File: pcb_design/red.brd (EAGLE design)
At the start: 160 x 100 mm, 6 parts, among them J1 4P-2.0, J2 4P-2.0

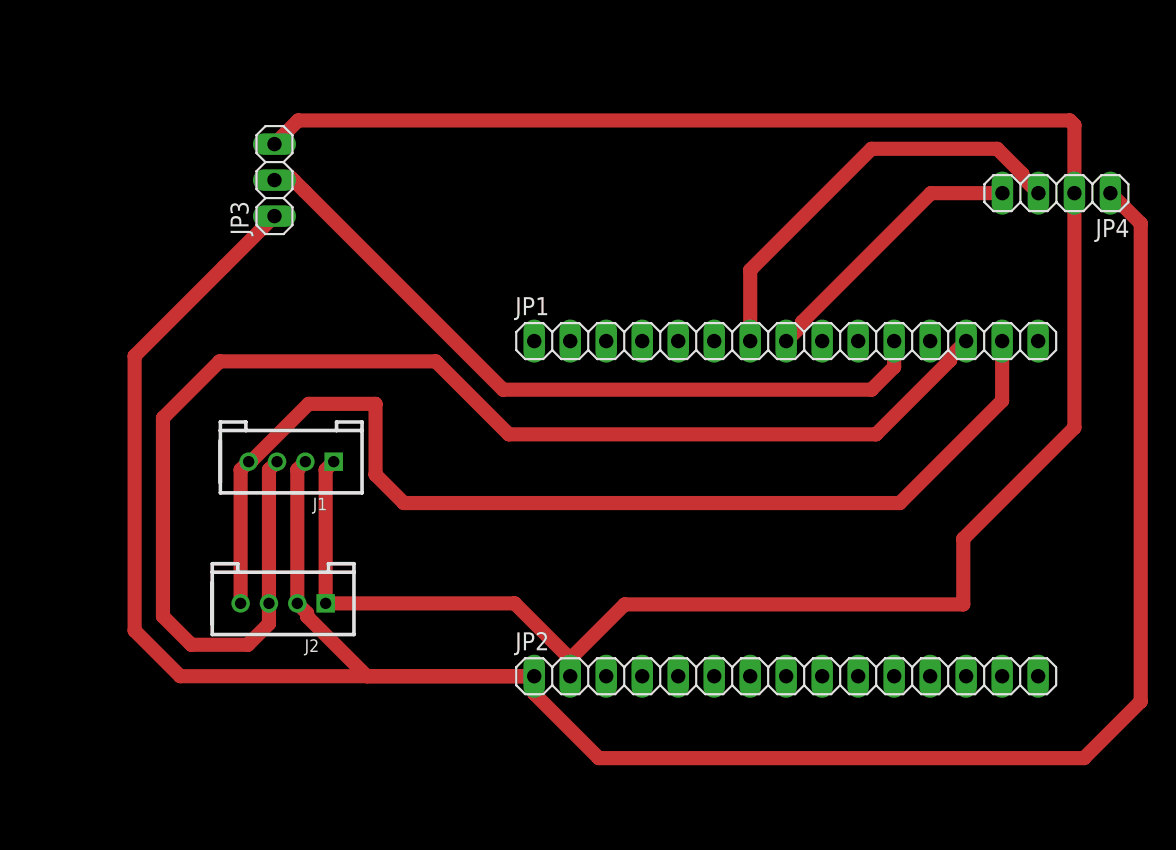
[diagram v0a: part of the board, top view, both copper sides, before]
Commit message: added latest combined data
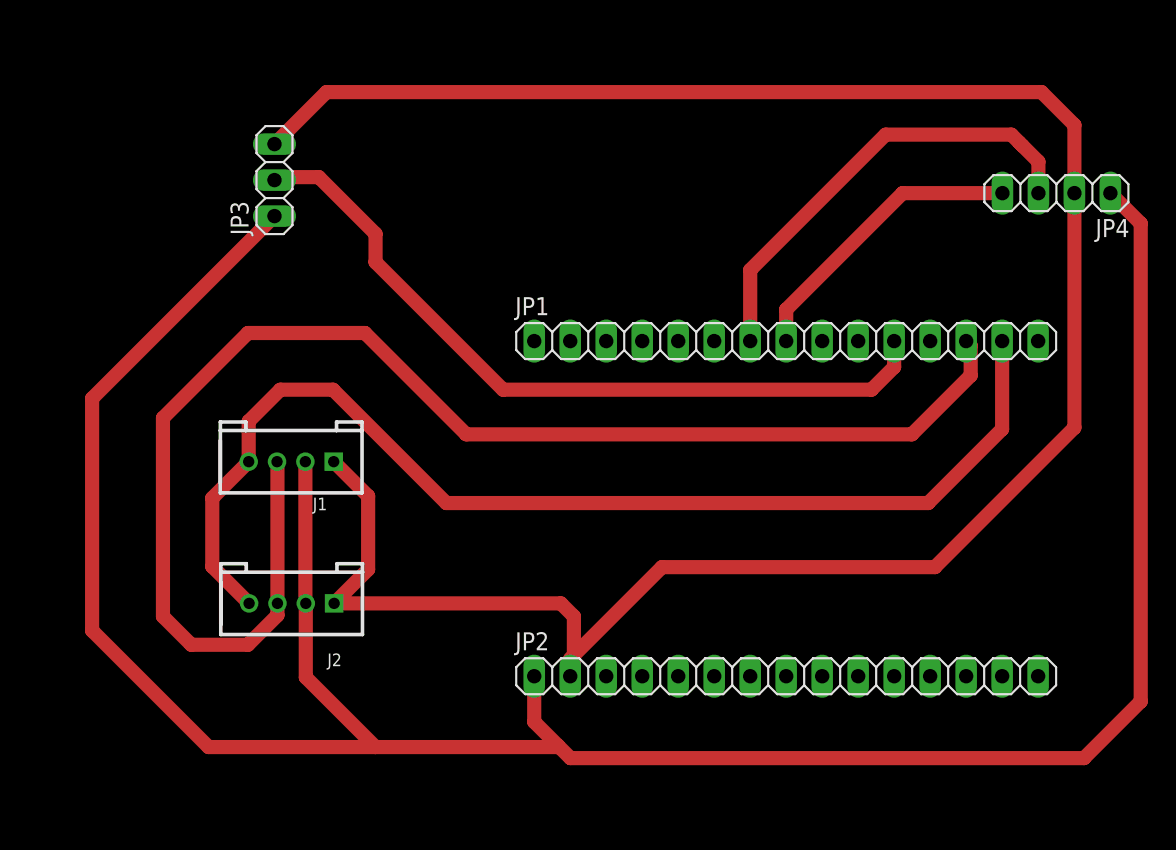
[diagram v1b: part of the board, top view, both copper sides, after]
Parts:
- moved J2 0.60 mm to (74.1, 30.9)
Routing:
- net N$8: track 98.1 -> 101.4 mm
- net N$7: track 78.1 -> 80.8 mm
- net N$9: track 155.2 -> 157.5 mm
- net N$6: track 176.4 -> 178.6 mm
- net N$5: track 30.3 -> 32.3 mm
- net N$4: track 19.7 -> 20.9 mm
- net N$3: track 52.6 -> 53.7 mm
